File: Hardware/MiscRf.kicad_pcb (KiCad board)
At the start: 2 copper layers, 38.1 x 45.7 mm, 15 parts, among them J1 SMA, J2 SMA, J3 SMA, J4 SMA, J5 SMA, U1 0915LP

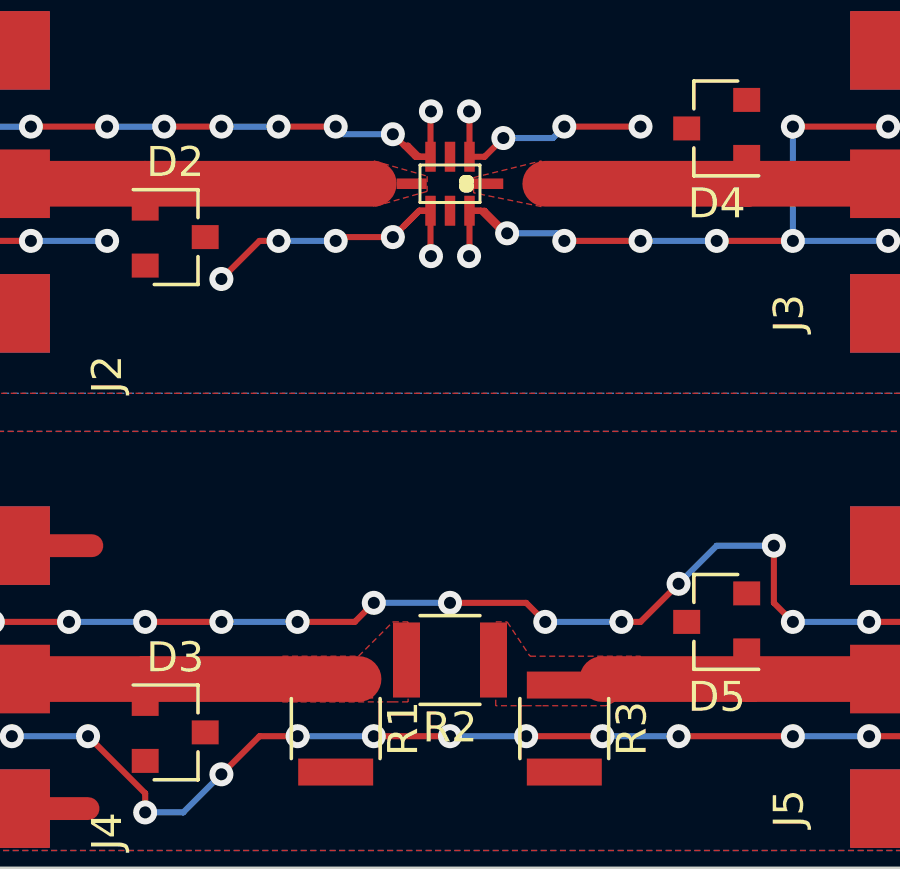
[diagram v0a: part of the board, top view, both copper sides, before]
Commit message: Generated Gerbers
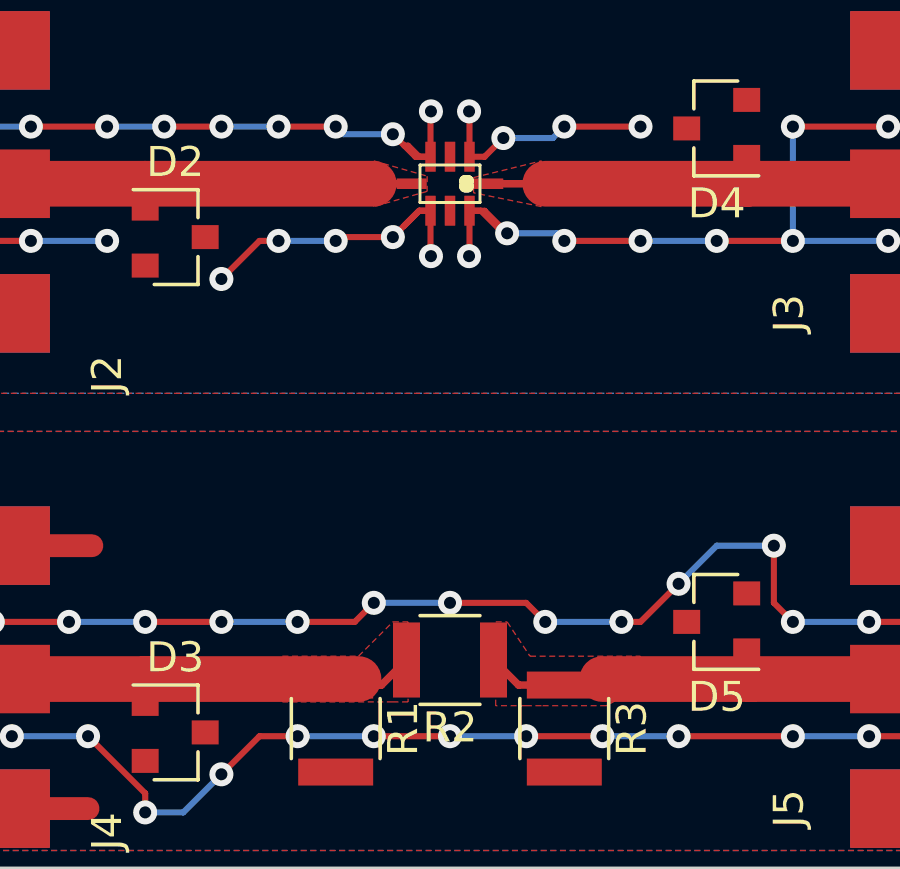
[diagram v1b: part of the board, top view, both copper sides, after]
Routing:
- net Net-(D3-Pad1): track 13.7 -> 16.4 mm
- net Net-(D5-Pad1): track 11.8 -> 14.5 mm
- net Net-(D4-Pad1): track 13.6 -> 15.5 mm
- net Net-(D2-Pad1): track 14.2 -> 15.4 mm
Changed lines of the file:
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@@
     (thickness 1.6)
     (drawings 5)
-    (tracks 209)
+    (tracks 215)
     (zones 0)
     (modules 15)
@@
       (padsonsilk false)
       (subtractmaskfromsilk false)
-      (outputformat 4)
+      (outputformat 1)
       (mirror false)
       (drillshape 0)
@@
   (segment (start 161.29 85.725) (end 165.227 85.725) (width 0.762) (layer F.Cu) (net 2))
   (segment (start 161.29 85.725) (end 161.29 82.931) (width 0.762) (layer F.Cu) (net 2))
+  (segment (start 175.89 73.66) (end 174.625 73.66) (width 0.25) (layer F.Cu) (net 3))
   (segment (start 167.005 74.488) (end 167.005 73.773) (width 0.762) (layer F.Cu) (net 3))
   (segment (start 161.29 73.66) (end 167.005 73.66) (width 1.524) (layer F.Cu) (net 3))
   (segment (start 167.005 73.66) (end 174.625 73.66) (width 1.524) (layer F.Cu) (net 3))
   (segment (start 167.005 73.773) (end 167.005 73.66) (width 0.762) (layer F.Cu) (net 3))
+  (segment (start 173.355 90.371) (end 174.879 90.371) (width 0.25) (layer F.Cu) (net 4))
+  (segment (start 174.879 90.371) (end 175.715 89.535) (width 0.25) (layer F.Cu) (net 4))
   (segment (start 161.29 90.17) (end 167.005 90.17) (width 1.524) (layer F.Cu) (net 4))
   (segment (start 167.005 90.17) (end 174.117 90.17) (width 1.524) (layer F.Cu) (net 4))
   (segment (start 167.005 90.998) (end 167.005 90.17) (width 0.762) (layer F.Cu) (net 4))
+  (segment (start 178.44 73.66) (end 180.34 73.66) (width 0.25) (layer F.Cu) (net 5))
   (segment (start 193.04 73.66) (end 187.071 73.66) (width 1.524) (layer F.Cu) (net 5))
   (segment (start 187.071 73.66) (end 180.34 73.66) (width 1.524) (layer F.Cu) (net 5))
   (segment (start 187.055 72.766) (end 187.055 73.644) (width 0.762) (layer F.Cu) (net 5))
   (segment (start 187.055 73.644) (end 187.071 73.66) (width 0.762) (layer F.Cu) (net 5))
+  (segment (start 180.975 90.371) (end 179.451 90.371) (width 0.25) (layer F.Cu) (net 6))
+  (segment (start 179.451 90.371) (end 178.615 89.535) (width 0.25) (layer F.Cu) (net 6))
   (segment (start 191.643 90.17) (end 187.198 90.17) (width 1.524) (layer F.Cu) (net 6))
   (segment (start 187.198 90.17) (end 182.245 90.17) (width 1.524) (layer F.Cu) (net 6))
